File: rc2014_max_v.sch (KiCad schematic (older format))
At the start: 30 parts, among them J1 M3 Mounting Hole, J2 Conn_01x40, J3 Conn_01x24, U1 TXB0108PWR, U2 TXB0108PWR, U3 TXB0108PWR, U4 TXB0108PWR, U5 TXB0108PWR, U6 TXB0108PWR, U7 TXB0108PWR

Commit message: Updated BOM
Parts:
- C1, C10, C11, C12, C13, C14, C15, C2, C3, C4, C5, C6, C7, C8, C9: MFR KEMET -> Taiyo Yuden; MPN C0805C104K4RACTU -> TMK107BJ104KA-T; SPN 80-C0805C104K4R -> (none)
- R1, R2, R3, R4: MFR (none) -> Yageo; MPN (none) -> RC0603JR-071KL; SPR (none) -> Mouser
- RN1: MFR (none) -> Panasonic; MPN (none) -> EXB-38V103JV; SPR (none) -> Mouser
- U1, U2, U3, U4, U5, U6, U7: MFR (none) -> Texas Instruments; MPN (none) -> TXB0108PWR; SPR (none) -> Mouser

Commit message: updated descriptions and part #'s
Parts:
- C1, C10, C11, C12, C13, C14, C15, C2, C3, C4, C5, C6, C7, C8, C9: Description (none) -> Multilayer Ceramic Capacitors MLCC - SMD/SMT 0.1uF 25V X5R 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; SPN (none) -> 963-TMK107BJ104KA-T; SPURL https://www.mouser.com/ProductDetail/KEMET/C0805C104K4RACTU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 -> https://www.mouser.com/ProductDetail/963-TMK107BJ104KA-T
- R1, R2, R3, R4: Description (none) -> Thick Film Resistors - SMD 1K OHM 5%; SPN (none) -> 603-RC0603JR-071KL; SPURL (none) -> https://www.mouser.com/ProductDetail/603-RC0603JR-071KL
- RN1: Description (none) -> Resistor Networks & Arrays 10K OHM 5%; SPN (none) -> 667-EXB-38V103JV; SPURL (none) -> https://www.mouser.com/ProductDetail/667-EXB-38V103JV
- U1, U2, U3, U4, U5, U6, U7: Description (none) -> Translation - Voltage Levels 8-Bit Bi-directional V-Level T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; SPN (none) -> 595-TXB0108PWR; SPURL (none) -> https://www.mouser.com/ProductDetail/595-TXB0108PWR

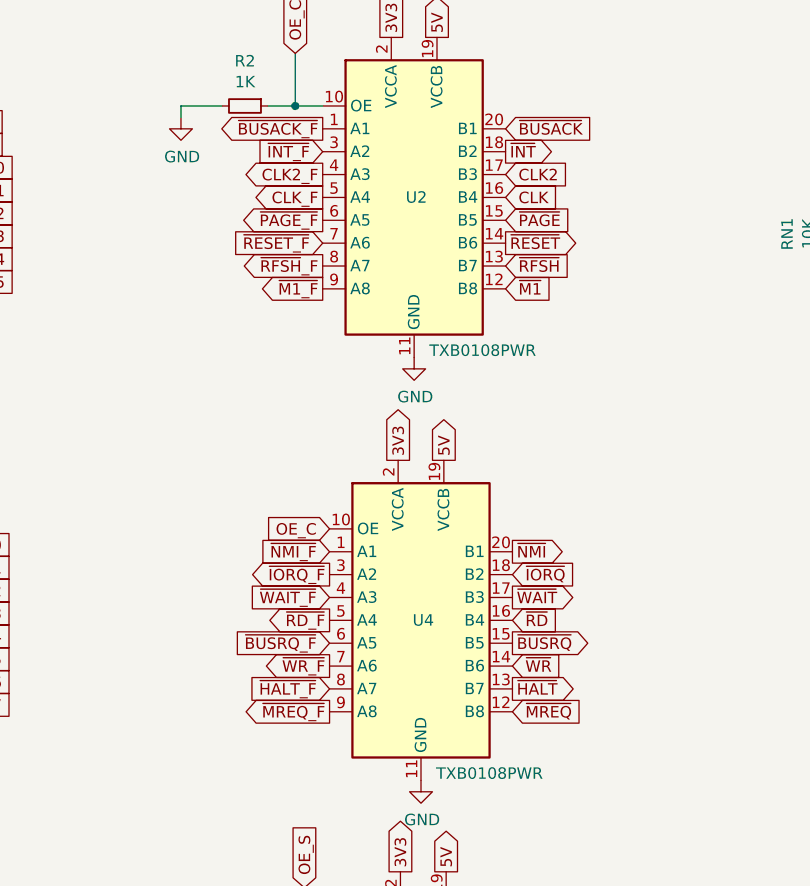
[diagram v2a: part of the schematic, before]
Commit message: parts placement
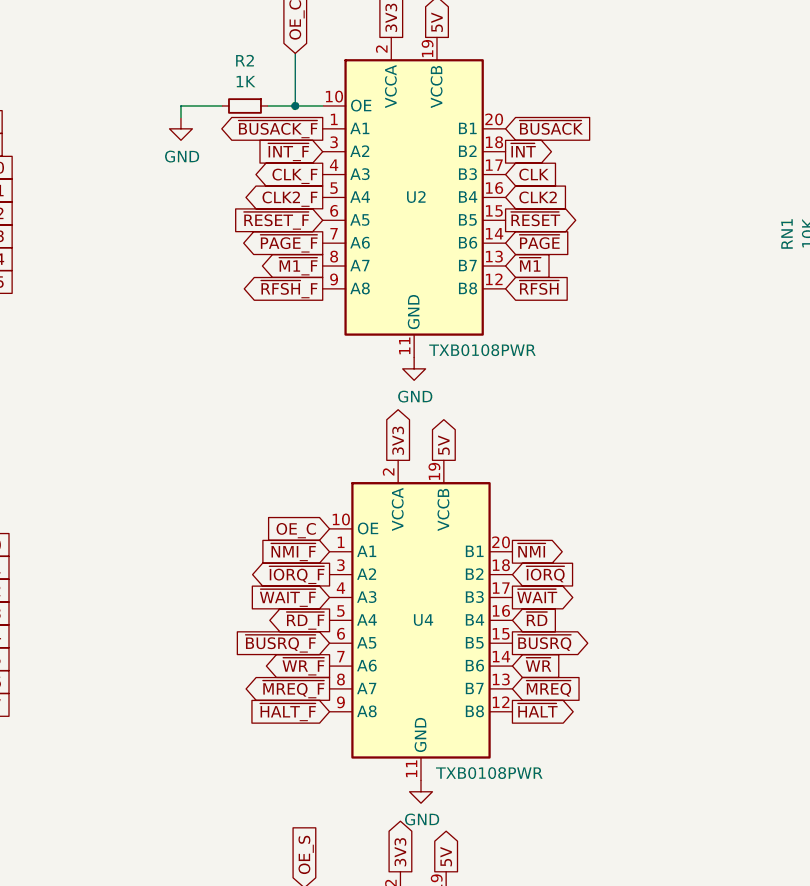
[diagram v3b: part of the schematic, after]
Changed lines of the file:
@@
 Text GLabel 870  5640 2    50   Input ~ 0
 RXA
-Text GLabel 5440 3680 0    50   Output ~ 0
+Text GLabel 5440 3580 0    50   Output ~ 0
 ~MREQ_F
 Text GLabel 5440 3480 0    50   Output ~ 0
@@
 Text GLabel 3890 7340 2    50   3State ~ 0
 D12
-Text GLabel 6240 3580 2    50   Output ~ 0
+Text GLabel 6240 3680 2    50   Output ~ 0
 ~HALT
 Text GLabel 6240 3380 2    50   Output ~ 0
@@
 Text GLabel 6210 1230 2    50   Output ~ 0
 ~INT
-Text GLabel 6210 1630 2    50   Output ~ 0
+Text GLabel 6210 1530 2    50   Output ~ 0
 ~RESET
 Text GLabel 6210 1130 2    50   Input ~ 0
 ~BUSACK
-Text GLabel 6210 1530 2    50   Input ~ 0
+Text GLabel 6210 1630 2    50   Input ~ 0
 ~PAGE
-Text GLabel 6240 3680 2    50   Input ~ 0
+Text GLabel 6240 3580 2    50   Input ~ 0
 ~MREQ
 Text GLabel 6240 3480 2    50   Input ~ 0
@@
 Text GLabel 6240 3080 2    50   Input ~ 0
 ~IORQ
-Text GLabel 6210 1830 2    50   Input ~ 0
+Text GLabel 6210 1730 2    50   Input ~ 0
 ~M1
-Text GLabel 6210 1430 2    50   Input ~ 0
+Text GLabel 6210 1330 2    50   Input ~ 0
 CLK
 Text GLabel 5440 2980 0    50   Input ~ 0
@@
 Text GLabel 5440 3380 0    50   Input ~ 0
 ~BUSRQ_F
-Text GLabel 5440 3580 0    50   Input ~ 0
+Text GLabel 5440 3680 0    50   Input ~ 0
 ~HALT_F
 Text GLabel 6250 4980 2    50   Input ~ 0
@@
 Text GLabel 5290 800  1    50   Input ~ 0
 OE_C
-Text GLabel 6210 1730 2    50   Input ~ 0
+Text GLabel 6210 1830 2    50   Input ~ 0
 ~RFSH
-Text GLabel 6210 1330 2    50   Input ~ 0
+Text GLabel 6210 1430 2    50   Input ~ 0
 CLK2
 Text GLabel 7960 1790 3    50   Output ~ 0
@@
 Text GLabel 7760 1790 3    50   Output ~ 0
 ~NMI
-Text GLabel 5410 1330 0    50   Output ~ 0
+Text GLabel 5410 1430 0    50   Output ~ 0
 CLK2_F
-Text GLabel 5410 1730 0    50   Output ~ 0
+Text GLabel 5410 1830 0    50   Output ~ 0
 ~RFSH~_F
 Text GLabel 5410 1230 0    50   Input ~ 0
 ~INT_F
-Text GLabel 5410 1630 0    50   Input ~ 0
+Text GLabel 5410 1530 0    50   Input ~ 0
 ~RESET_F
-Text GLabel 5410 1430 0    50   Output ~ 0
+Text GLabel 5410 1330 0    50   Output ~ 0
 CLK_F
-Text GLabel 5410 1830 0    50   Output ~ 0
+Text GLabel 5410 1730 0    50   Output ~ 0
 ~M1_F
-Text GLabel 5410 1530 0    50   Output ~ 0
+Text GLabel 5410 1630 0    50   Output ~ 0
 ~PAGE_F
 Text GLabel 5410 1130 0    50   Output ~ 0

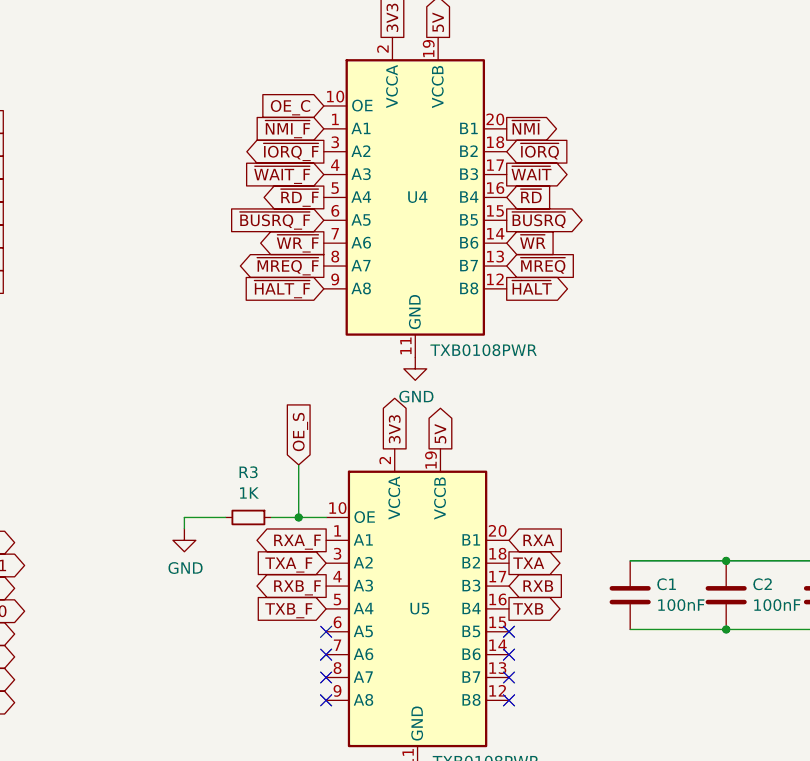
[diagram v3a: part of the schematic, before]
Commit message: started routing
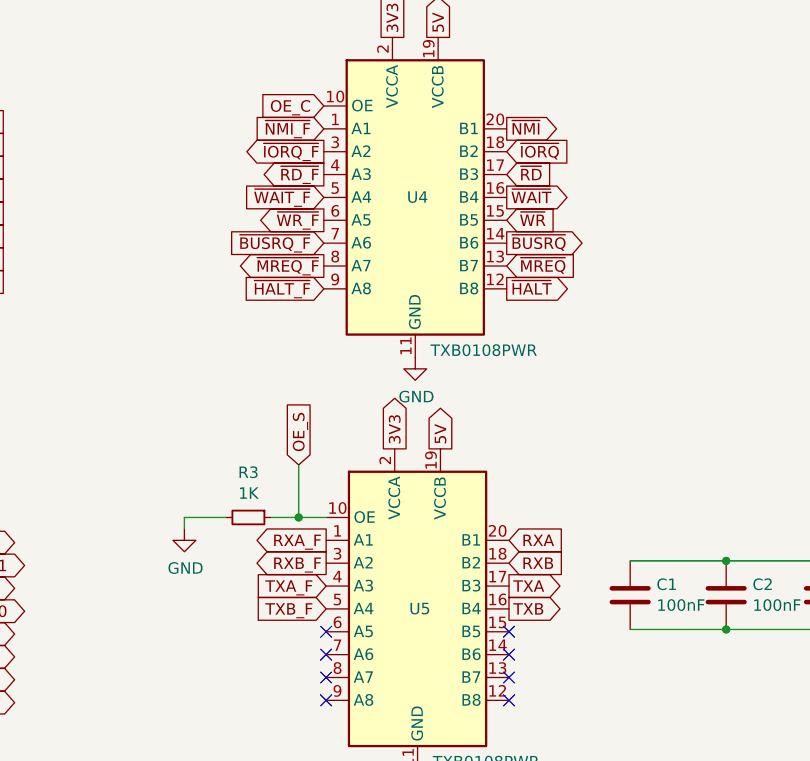
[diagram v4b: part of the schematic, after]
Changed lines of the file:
@@
 Text GLabel 5440 3580 0    50   Output ~ 0
 ~MREQ_F
-Text GLabel 5440 3480 0    50   Output ~ 0
+Text GLabel 5440 3380 0    50   Output ~ 0
 ~WR_F
-Text GLabel 5440 3280 0    50   Output ~ 0
+Text GLabel 5440 3180 0    50   Output ~ 0
 ~RD_F
 Text GLabel 5440 3080 0    50   Output ~ 0
@@
 Text GLabel 6240 3680 2    50   Output ~ 0
 ~HALT
-Text GLabel 6240 3380 2    50   Output ~ 0
+Text GLabel 6240 3480 2    50   Output ~ 0
 ~BUSRQ
-Text GLabel 6240 3180 2    50   Output ~ 0
+Text GLabel 6240 3280 2    50   Output ~ 0
 ~WAIT
 Text GLabel 6240 2980 2    50   Output ~ 0
@@
 Text GLabel 6240 3580 2    50   Input ~ 0
 ~MREQ
-Text GLabel 6240 3480 2    50   Input ~ 0
+Text GLabel 6240 3380 2    50   Input ~ 0
 ~WR
-Text GLabel 6240 3280 2    50   Input ~ 0
+Text GLabel 6240 3180 2    50   Input ~ 0
 ~RD
 Text GLabel 6240 3080 2    50   Input ~ 0
@@
 Text GLabel 5440 2980 0    50   Input ~ 0
 ~NMI_F
-Text GLabel 5440 3180 0    50   Input ~ 0
+Text GLabel 5440 3280 0    50   Input ~ 0
 ~WAIT_F
-Text GLabel 5440 3380 0    50   Input ~ 0
+Text GLabel 5440 3480 0    50   Input ~ 0
 ~BUSRQ_F
 Text GLabel 5440 3680 0    50   Input ~ 0
 ~HALT_F
-Text GLabel 6250 4980 2    50   Input ~ 0
+Text GLabel 6250 4880 2    50   Input ~ 0
 RXB
 Text GLabel 6250 5080 2    50   Output ~ 0
@@
 Text GLabel 6250 4780 2    50   Input ~ 0
 RXA
-Text GLabel 6250 4880 2    50   Output ~ 0
+Text GLabel 6250 4980 2    50   Output ~ 0
 TXA
 Text GLabel 5450 4780 0    50   Output ~ 0
 RXA_F
-Text GLabel 5450 4880 0    50   Input ~ 0
+Text GLabel 5450 4980 0    50   Input ~ 0
 TXA_F
-Text GLabel 5450 4980 0    50   Output ~ 0
+Text GLabel 5450 4880 0    50   Output ~ 0
 RXB_F
 Text GLabel 5450 5080 0    50   Input ~ 0
